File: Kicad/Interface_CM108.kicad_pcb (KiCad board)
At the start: 2 copper layers, 76 x 51 mm, 43 parts, among them IC1 CM108B, J1 USB_C_Receptacle_USB2.0_16P, J2 RJ45, Q1 BC546ABU, T1 Transformer_1P_1S, T2 Transformer_1P_1S, U1 93C46, U2 PC318

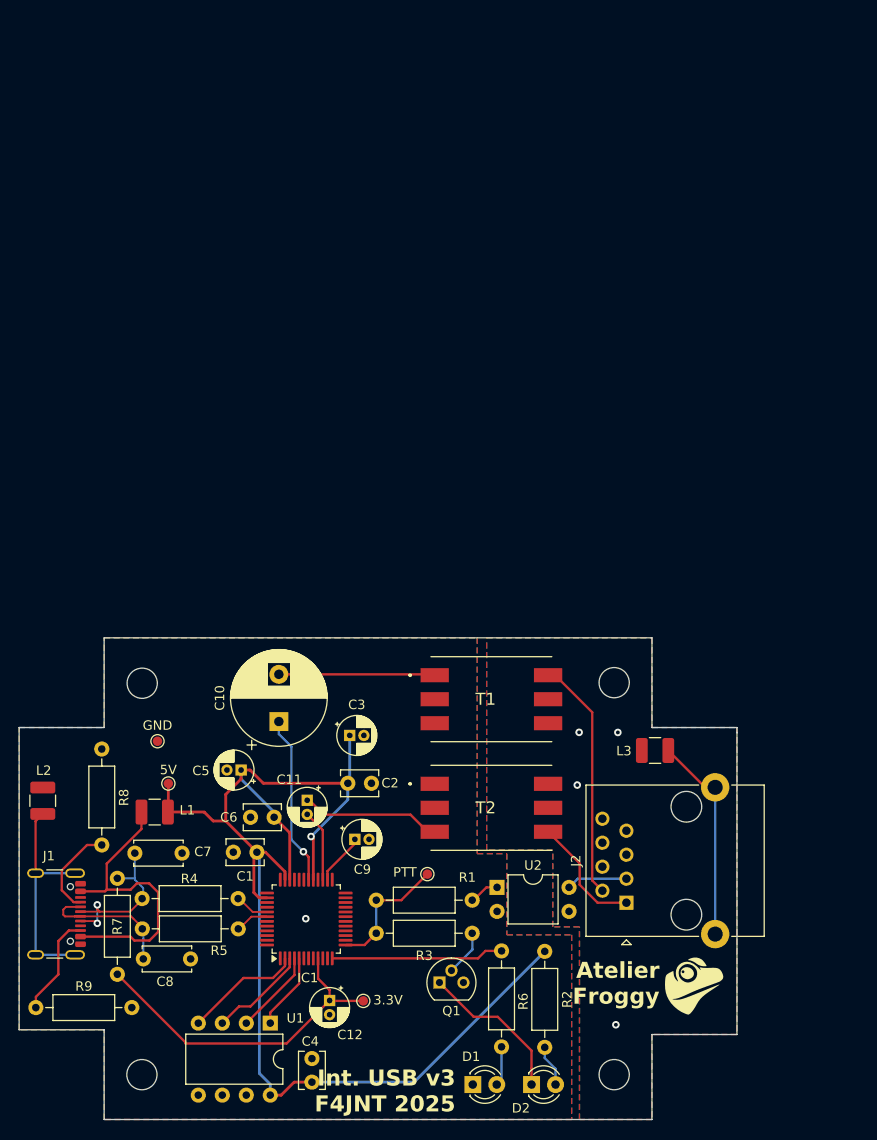
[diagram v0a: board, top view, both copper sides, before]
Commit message: Revision v4
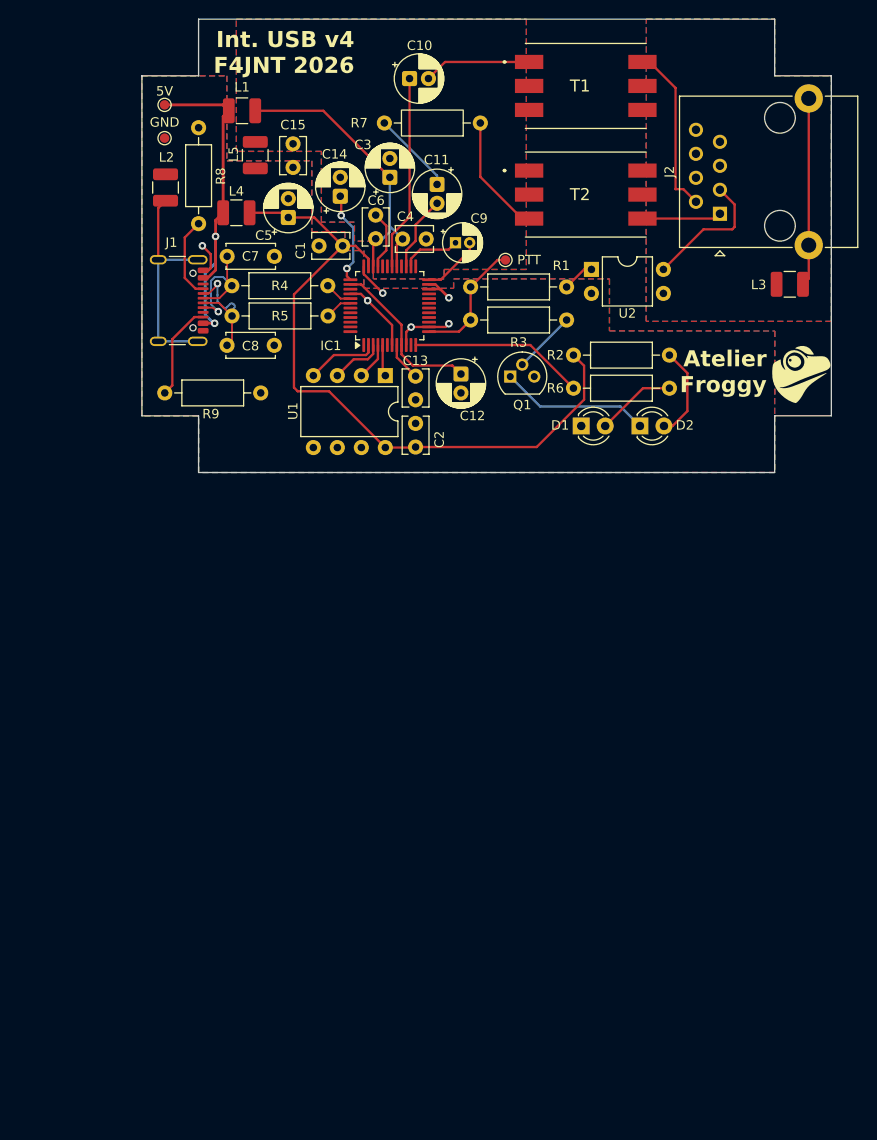
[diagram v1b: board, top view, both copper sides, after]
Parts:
- removed 3.3V: 3.3V, TestPoint:TestPoint_Pad_D1.0mm
- removed vis1, vis2, vis3, vis4: MountingHole_3.2mm_M3, MountingHole:MountingHole_3.2mm_M3
- added C13: 100nF, Capacitor_THT:C_Disc_D3.8mm_W2.6mm_P2.50mm, F.Cu at (98.5, 75.3)
- added C14: 10µ, Capacitor_THT:CP_Radial_D5.0mm_P2.00mm, F.Cu at (90.5, 53.8)
- added C15: 10µF, Capacitor_THT:C_Disc_D3.8mm_W2.6mm_P2.50mm, F.Cu at (85.5, 50.7)
- added L4: Ferrite_Bead, Inductor_SMD:L_1210_3225Metric, F.Cu at (79.5, 55.5)
- added L5: Ferrite_Bead, Inductor_SMD:L_1210_3225Metric, F.Cu at (81.5, 49.4)
- C10: value 470μ -> 100μF; footprint Capacitor_THT:CP_Radial_D10.0mm_P5.00mm -> Capacitor_THT:CP_Radial_D5.0mm_P2.00mm
- C11: value 1µ -> 1µF; footprint Capacitor_THT:CP_Radial_D4.0mm_P1.50mm -> Capacitor_THT:CP_Radial_D5.0mm_P2.00mm
- C12: value 4.7µ -> 1µF; footprint Capacitor_THT:CP_Radial_D4.0mm_P1.50mm -> Capacitor_THT:CP_Radial_D5.0mm_P2.00mm
- C3, C5: value 4.7µ -> 10µ; footprint Capacitor_THT:CP_Radial_D4.0mm_P1.50mm -> Capacitor_THT:CP_Radial_D5.0mm_P2.00mm
- R4, R5: value 22 -> 39
- R7: value 1.5k -> 8.2k
- moved R7 98.0 mm to (105.3, 46.0), turned to 180 degrees
- moved C4 89.8 mm to (97.1, 58.3), turned to 0 degrees
- moved L1 74.8 mm to (80.1, 44.7)
- moved J2 73.6 mm to (130.7, 55.6)
- moved R6 72.0 mm to (125.3, 74.1), turned to 180 degrees
- moved 5V 71.9 mm to (71.9, 44.1)
- moved D1 70.7 mm to (116.0, 78.1)
- moved D2 70.7 mm to (122.2, 78.1)
- moved U1 69.6 mm to (95.3, 72.7)
- moved C10 69.5 mm to (97.8, 41.3), turned to 0 degrees
- moved C12 67.8 mm to (103.3, 72.6)
- moved C11 66.6 mm to (100.8, 52.5)
- moved R8 66.6 mm to (75.5, 46.5)
- moved R9 66.5 mm to (82.1, 74.6)
- moved J1 66.2 mm to (72.3, 64.8)
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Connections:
- C1 pad 1: VBUS -> +5VD
- C1 pad 2: GND -> GNDD
- C11 pad 1: /MIC_IN -> Net-(C11-Pad1)
- C12 pad 1: +3.3V -> +3V3
- C12 pad 2: GND -> GNDD
- C2 pad 1: VBUS -> +5VD
- C2 pad 2: GND -> GNDD
- C3 pad 1: VBUS -> +5VA
- C3 pad 2: GND -> GNDA
- C4 pad 1: VBUS -> +5VA
- C4 pad 2: GND -> GNDA
- C5 pad 1: VBUS -> +5VD
- C5 pad 2: GND -> GNDD
- C6 pad 1: VBUS -> +5VA
- C6 pad 2: GND -> GNDA
- C7 pad 2: GND -> GNDD
- C8 pad 2: GND -> GNDD
- C9 pad 2: GND -> GNDA
- D1 pad 1: GND -> GNDD
- GND pad 1: GND -> GNDD
- IC1 pad 10: GND -> GNDD
- IC1 pad 14: GND -> GNDD
- IC1 pad 22: GND -> GNDD
- IC1 pad 23: GND -> GNDD
- IC1 pad 24: GND -> GNDA
- IC1 pad 29: VBUS -> +5VA
- IC1 pad 33: GND -> GNDA
- IC1 pad 34: VBUS -> +5VA
- IC1 pad 35: VBUS -> +5VD
- IC1 pad 36: GND -> GNDD
- IC1 pad 37: unconnected-(IC1-AREG36-Pad37) -> Net-(IC1-AREG36)
- IC1 pad 38: VBUS -> +3V3
- IC1 pad 40: GND -> GNDD
- IC1 pad 7: GND -> GNDD
- IC1 pad 8: unconnected-(IC1-DREG18-Pad8) -> Net-(IC1-DREG18)
- IC1 pad 9: +3.3V -> +3V3
- J1 pad A1: GND -> GNDD
- J1 pad A12: GND -> GNDD
- J1 pad A4: Net-(J1-VBUS-PadA4) -> VBUS
- J1 pad A9: Net-(J1-VBUS-PadA4) -> VBUS
- J1 pad B1: GND -> GNDD
- J1 pad B12: GND -> GNDD
- J1 pad B4: Net-(J1-VBUS-PadA4) -> VBUS
- J1 pad B9: Net-(J1-VBUS-PadA4) -> VBUS
- L1 pad 1: Net-(J1-VBUS-PadA4) -> VBUS
- L1 pad 2: VBUS -> +5VA
- L2 pad 1: GND -> GNDD
- Q1 pad 3: GND -> GNDD
- R2 pad 1: VBUS -> +5VD
- R7 pad 1: +3.3V -> /MIC_IN
- R7 pad 2: /USB+ -> Net-(C11-Pad1)
- R8 pad 1: GND -> GNDD
- R9 pad 1: GND -> GNDD
- T1 pad 3: GND -> GNDA
- T2 pad 1: GND -> GNDA
- U1 pad 5: GND -> GNDD
- U1 pad 8: VBUS -> +5VD
- U2 pad 2: GND -> GNDD
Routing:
- net VBUS: track 135.4 -> 37.5 mm, vias 1 -> 2
- net +5VD: track 0.00 -> 73.2 mm
- net +3.3V: track 36.0 -> 0.00 mm
- net +5VA: track 0.00 -> 32.8 mm
- net Net-(J1-VBUS-PadA4): track 31.7 -> 0.00 mm
- net GNDD: track 0.00 -> 26.6 mm, vias 0 -> 6
- net +3V3: track 0.00 -> 17.5 mm
- net GNDA: track 0.00 -> 12.7 mm
- net Net-(IC1-AREG36): track 0.00 -> 9.84 mm, vias 0 -> 2
- net Net-(C11-Pad1): track 0.00 -> 8.81 mm
- net /RADIO_MIC: track 25.6 -> 18.1 mm
- net /RADIO_PTT: track 6.46 -> 14.0 mm
- net Net-(D2-A): track 4.41 -> 9.85 mm
- net /AUDIO_L: track 16.5 -> 11.4 mm
- net /SCLK: track 8.97 -> 3.96 mm
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- added copper zone on B.Cu, net GNDA
- added copper zone on F.Cu, net GNDA
- added copper zone on B.Cu, net GNDD
- added copper zone on F.Cu, net GNDD
- removed copper zone on B.Cu, net GND
- removed copper zone on F.Cu, net GND
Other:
- board size 76 x 51 mm -> 73 x 48 mm
- board text added: "Int. USB v4 F4JNT 2026"
- board text removed: "Int. USB v3 F4JNT 2025"
